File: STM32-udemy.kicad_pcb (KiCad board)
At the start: 2 copper layers, 66 x 26 mm, 27 parts, among them J2 Serial_Wire, J3 Conn_01x20_Male, J4 Conn_01x20_Male, SW1 SW_Push, SW2 SW_SPDT, U2 STM32F446RCTx, Y1 Crystal_GND24

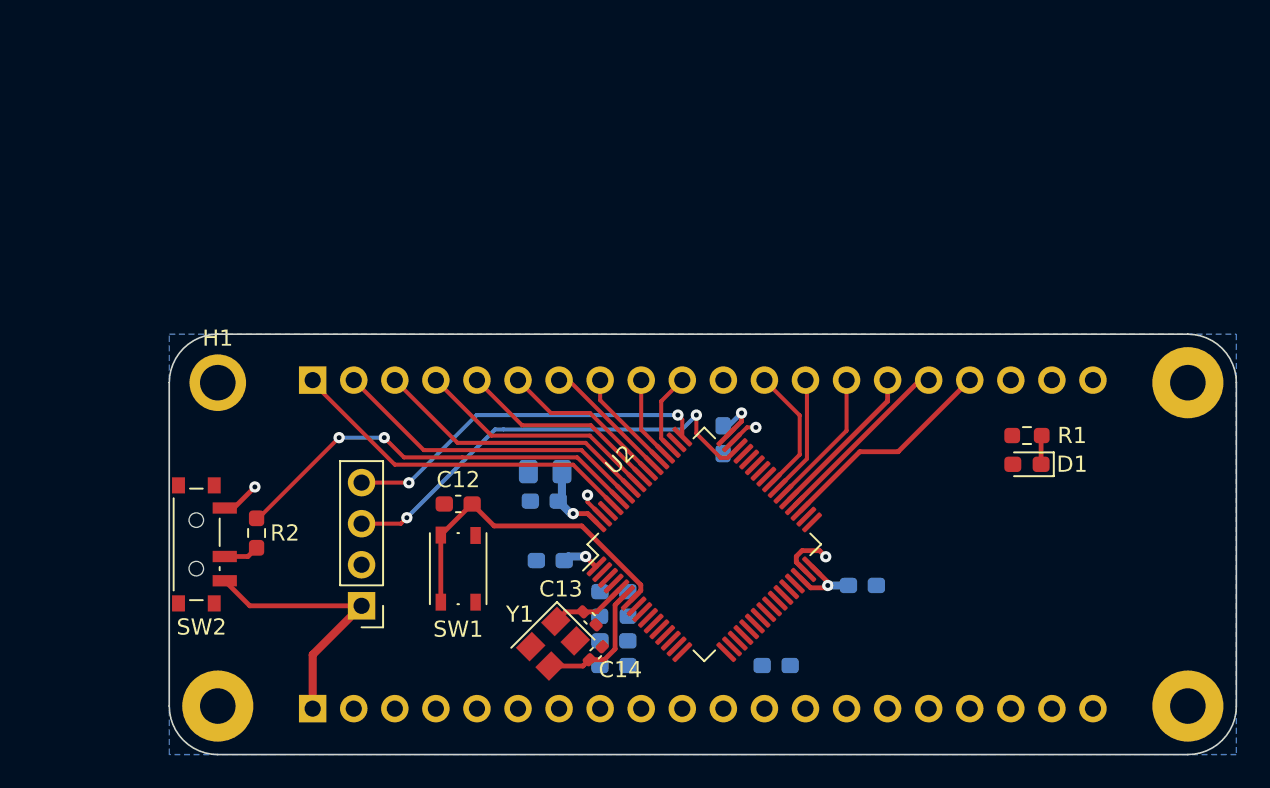
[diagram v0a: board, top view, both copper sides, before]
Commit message: Initial board layout
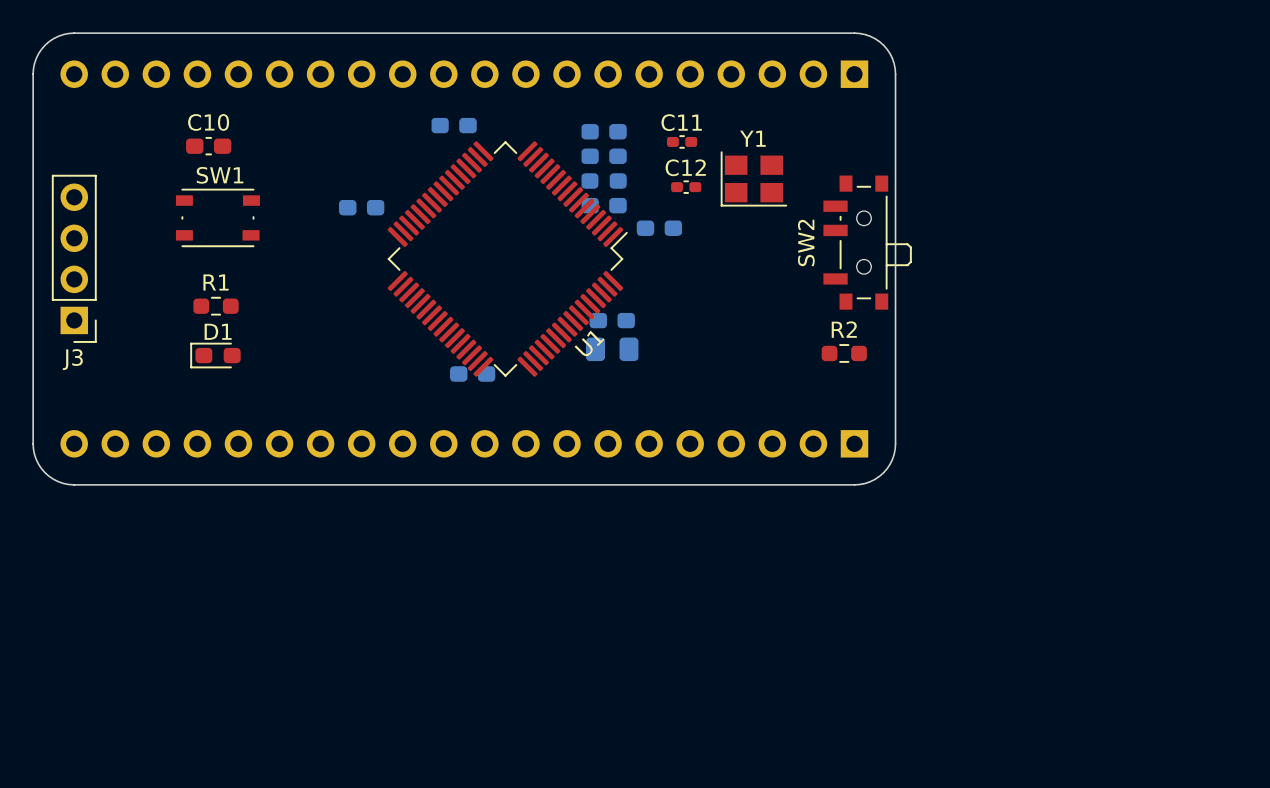
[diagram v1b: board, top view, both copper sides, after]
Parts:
- removed C13, C14: C, Capacitor_SMD:C_0402_1005Metric_Pad0.74x0.62mm_HandSolder
- removed H1: MountingHole, MountingHole:MountingHole_2.2mm_M2_ISO7380_Pad
- removed H2, H3, H4: MountingHole, MountingHole:MountingHole_2.2mm_M2_Pad
- removed J4: Conn_01x20_Male, Connector_PinHeader_2.54mm:PinHeader_1x20_P2.54mm_Vertical
- removed U2: STM32F446RCTx, Package_QFP:LQFP-64_10x10mm_P0.5mm
- added C1: 10u, Capacitor_SMD:C_0805_2012Metric_Pad1.18x1.45mm_HandSolder, B.Cu at (104.4, 75.4)
- added C2: 100n, Capacitor_SMD:C_0603_1608Metric_Pad1.08x0.95mm_HandSolder, B.Cu at (104.4, 73.7)
- added J1: Conn_01x20_Male, Connector_PinHeader_2.54mm:PinHeader_1x20_P2.54mm_Vertical, B.Cu at (119.4, 58.4)
- added U1: STM32F446RCTx, Package_QFP:LQFP-64_10x10mm_P0.5mm, F.Cu at (97.8, 69.8)
- C10: value 1u -> 100n; moved to F.Cu
- C11: value 1u -> C; footprint Capacitor_SMD:C_0603_1608Metric_Pad1.08x0.95mm_HandSolder -> Capacitor_SMD:C_0402_1005Metric_Pad0.74x0.62mm_HandSolder; moved to F.Cu
- C12: value 100n -> C; footprint Capacitor_SMD:C_0603_1608Metric_Pad1.08x0.95mm_HandSolder -> Capacitor_SMD:C_0402_1005Metric_Pad0.74x0.62mm_HandSolder
- C3: value 10u -> 100n; footprint Capacitor_SMD:C_0805_2012Metric_Pad1.18x1.45mm_HandSolder -> Capacitor_SMD:C_0603_1608Metric_Pad1.08x0.95mm_HandSolder
- C8, C9: value 100n -> 1u
- J2: value Serial_Wire -> Conn_01x20_Male; footprint Connector_PinHeader_2.54mm:PinHeader_1x04_P2.54mm_Vertical -> Connector_PinHeader_2.54mm:PinHeader_1x20_P2.54mm_Vertical; moved to B.Cu
- J3: value Conn_01x20_Male -> Serial_Wire; footprint Connector_PinHeader_2.54mm:PinHeader_1x20_P2.54mm_Vertical -> Connector_PinHeader_2.54mm:PinHeader_1x04_P2.54mm_Vertical; moved to F.Cu
- moved R1 50.8 mm to (79.9, 72.8), turned to 0 degrees
- moved D1 50.5 mm to (80.0, 75.8), turned to 0 degrees
- moved SW2 44.7 mm to (119.6, 68.8), turned to 90 degrees
- moved C10 40.7 mm to (79.4, 62.9), turned to 0 degrees
- moved R2 38.0 mm to (118.8, 75.7), turned to 0 degrees
- moved C7 34.7 mm to (103.9, 62.0)
- moved J2 32.1 mm to (119.4, 81.3), turned to 90 degrees
- moved Y1 31.3 mm to (113.2, 64.9), turned to 0 degrees
- moved J3 28.2 mm to (71.1, 73.7), turned to 180 degrees
- moved C11 28.1 mm to (108.7, 62.6)
- moved C9 26.9 mm to (103.9, 66.5), turned to 0 degrees
- moved FB1 26.9 mm to (103.9, 65.0)
- moved SW1 26.3 mm to (80.0, 67.3), turned to 0 degrees
- moved C5 25.6 mm to (94.6, 61.6), turned to 180 degrees
- moved C6 25.4 mm to (107.3, 67.9), turned to 180 degrees
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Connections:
- C10 pad 1: +3.3VA -> /NRST
- C11 pad 1: +3V3 -> /HSE_IN
- C12 pad 1: /NRST -> /HSE_OUT
- C7 pad 1: +3V3 -> +3.3VA
- C8 pad 1: +3V3 -> +3.3VA
- C9 pad 1: +3.3VA -> +3V3
- J2 pad 1: +3V3 -> /PB8
- J2 pad 2: GND -> /PB7
- J2 pad 3: /SWDIO -> /PB6
- J2 pad 4: /SWCLK -> /PB5
- J3 pad 2: /PC13 -> GND
- J3 pad 3: /PC14 -> /SWDIO
- J3 pad 4: /PC15 -> /SWCLK
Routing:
- net +3V3: track 32.1 -> 0.00 mm, vias 4 -> 0
- net /SWDIO: track 28.1 -> 0.00 mm, vias 2 -> 0
- net /BOOT0: track 26.1 -> 0.00 mm, vias 2 -> 0
- net /SWCLK: track 22.8 -> 0.00 mm, vias 2 -> 0
- net /PB8: track 21.9 -> 0.00 mm
- net /NRST: track 20.6 -> 0.00 mm
- net /PB7: track 19.7 -> 0.00 mm
- net /PB6: track 17.4 -> 0.00 mm
- net /PB5: track 15.0 -> 0.00 mm
- net /PB14: track 13.8 -> 0.00 mm
- net /PB4: track 12.7 -> 0.00 mm
- net /PB15: track 11.5 -> 0.00 mm
- net /PB3: track 10.4 -> 0.00 mm
- net /PC6: track 9.91 -> 0.00 mm
- net GND: track 9.33 -> 0.00 mm, vias 4 -> 0
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- removed copper zone on B.Cu, net GND
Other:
- board size 66 x 26 mm -> 53.3 x 27.9 mm
